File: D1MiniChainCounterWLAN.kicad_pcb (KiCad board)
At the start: 2 copper layers, 74.9 x 50.2 mm, 20 parts, among them J1 Power, J2 D24V10F5, J3 Chain Sens., J4 Chain Sw., K1 G5Q-1A, K2 G5Q-1A, Q1 BC337, Q2 BC337, Q3 BC337, Q4 BC337, U1 WeMos_D1_mini, U2 H11L1

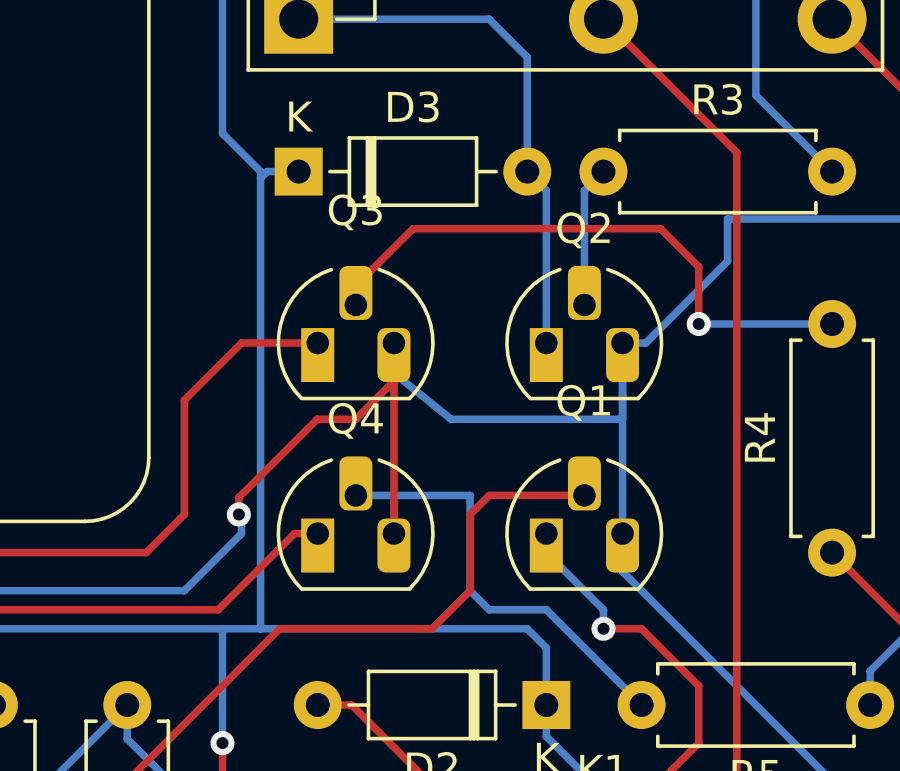
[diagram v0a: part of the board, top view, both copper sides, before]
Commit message: Version 1.1
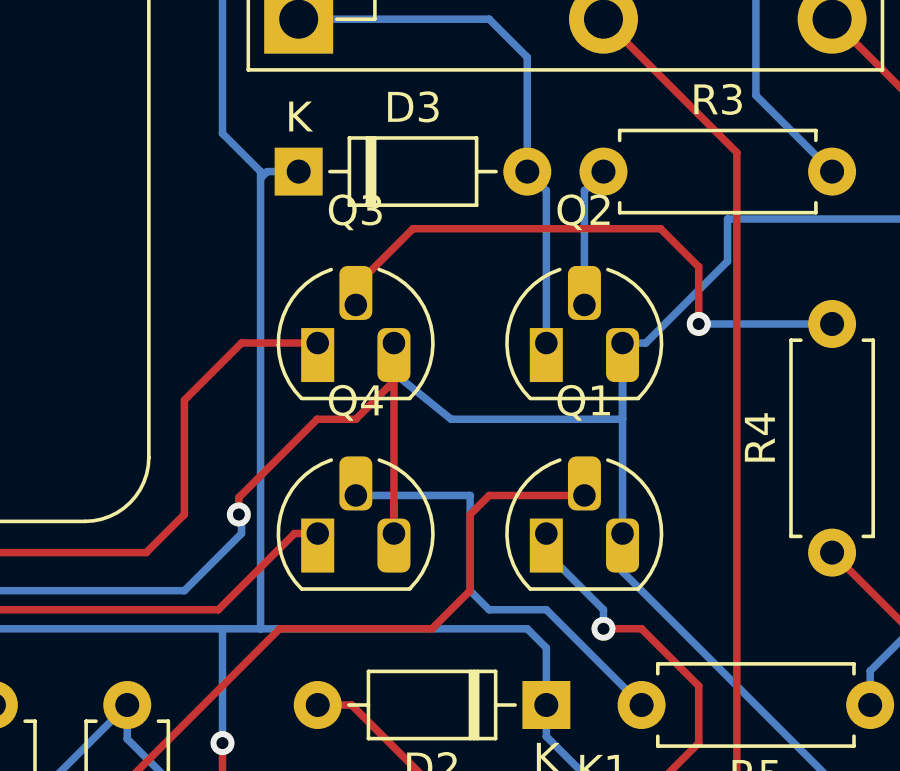
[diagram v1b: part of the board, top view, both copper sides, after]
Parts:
- Q2, Q4: footprint Package_TO_SOT_THT:TO-92L_HandSolder -> Package_TO_SOT_THT:TO-92_HandSolder
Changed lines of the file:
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@@
+  )
+  (module Package_TO_SOT_THT:TO-92_HandSolder (layer F.Cu)
+    (at 137.16 76.835)
+    (descr "TO-92 leads molded, narrow, drill 0.75mm, handsoldering variant with enlarged pads (see NXP sot054_po.pdf)")
+    (tags "to-92 sc-43 sc-43a sot54 PA33 transistor")
+    (fp_text reference Q4 (at 1.27 -4.4) (layer F.SilkS)
+      (effects (font (size 1 1) (thickness 0.15)))
+    )
+    (fp_text value BC337 (at 1.27 2.79) (layer F.Fab)
+      (effects (font (size 1 1) (thickness 0.15)))
+    )
+    (fp_arc (start 1.27 0) (end 2.05 -2.45) (angle 117.6433766) (layer F.SilkS) (width 0.12))
+    (fp_arc (start 1.27 0) (end 1.27 -2.48) (angle -135) (layer F.Fab) (width 0.1))
+    (fp_arc (start 1.27 0) (end 0.45 -2.45) (angle -116.9632683) (layer F.SilkS) (width 0.12))
+    (fp_arc (start 1.27 0) (end 1.27 -2.48) (angle 135) (layer F.Fab) (width 0.1))
+    (fp_line (start 4 2.01) (end -1.46 2.01) (layer F.CrtYd) (width 0.05))
+    (fp_line (start 4 2.01) (end 4 -3.05) (layer F.CrtYd) (width 0.05))
+    (fp_line (start -1.45 -3.05) (end -1.46 2.01) (layer F.CrtYd) (width 0.05))
+    (fp_line (start -1.46 -3.05) (end 4 -3.05) (layer F.CrtYd) (width 0.05))
+    (fp_line (start -0.5 1.75) (end 3 1.75) (layer F.Fab) (width 0.1))
+    (fp_line (start -0.53 1.85) (end 3.07 1.85) (layer F.SilkS) (width 0.12))
+    (fp_text user %R (at 1.27 -4.4) (layer F.Fab)
+      (effects (font (size 1 1) (thickness 0.15)))
+    )
+    (pad 1 thru_hole rect (at 0 0) (size 1.1 1.8) (drill 0.75 (offset 0 0.4)) (layers *.Cu *.Mask)
+      (net 11 "Net-(Q4-Pad1)"))
+    (pad 3 thru_hole roundrect (at 2.54 0) (size 1.1 1.8) (drill 0.75 (offset 0 0.4)) (layers *.Cu *.Mask) (roundrect_rratio 0.25)
+      (net 18 GND))
+    (pad 2 thru_hole roundrect (at 1.27 -1.27) (size 1.1 1.8) (drill 0.75 (offset 0 -0.4)) (layers *.Cu *.Mask) (roundrect_rratio 0.25)
+      (net 12 "Net-(Q4-Pad2)"))
+    (model ${KISYS3DMOD}/Package_TO_SOT_THT.3dshapes/TO-92.wrl
+      (at (xyz 0 0 0))
+      (scale (xyz 1 1 1))
+      (rotate (xyz 0 0 0))
+    )
+  )
+  (module Package_TO_SOT_THT:TO-92_HandSolder (layer F.Cu)
+    (at 144.78 70.485)
+    (descr "TO-92 leads molded, narrow, drill 0.75mm, handsoldering variant with enlarged pads (see NXP sot054_po.pdf)")
+    (tags "to-92 sc-43 sc-43a sot54 PA33 transistor")
+    (fp_text reference Q2 (at 1.27 -4.4) (layer F.SilkS)
+      (effects (font (size 1 1) (thickness 0.15)))
+    )
+    (fp_text value BC337 (at 1.27 2.79) (layer F.Fab)
+      (effects (font (size 1 1) (thickness 0.15)))
+    )
+    (fp_arc (start 1.27 0) (end 2.05 -2.45) (angle 117.6433766) (layer F.SilkS) (width 0.12))
+    (fp_arc (start 1.27 0) (end 1.27 -2.48) (angle -135) (layer F.Fab) (width 0.1))
+    (fp_arc (start 1.27 0) (end 0.45 -2.45) (angle -116.9632683) (layer F.SilkS) (width 0.12))
+    (fp_arc (start 1.27 0) (end 1.27 -2.48) (angle 135) (layer F.Fab) (width 0.1))
+    (fp_line (start 4 2.01) (end -1.46 2.01) (layer F.CrtYd) (width 0.05))
+    (fp_line (start 4 2.01) (end 4 -3.05) (layer F.CrtYd) (width 0.05))
+    (fp_line (start -1.45 -3.05) (end -1.46 2.01) (layer F.CrtYd) (width 0.05))
+    (fp_line (start -1.46 -3.05) (end 4 -3.05) (layer F.CrtYd) (width 0.05))
+    (fp_line (start -0.5 1.75) (end 3 1.75) (layer F.Fab) (width 0.1))
+    (fp_line (start -0.53 1.85) (end 3.07 1.85) (layer F.SilkS) (width 0.12))
+    (fp_text user %R (at 1.27 -4.4) (layer F.Fab)
+      (effects (font (size 1 1) (thickness 0.15)))
+    )
+    (pad 1 thru_hole rect (at 0 0) (size 1.1 1.8) (drill 0.75 (offset 0 0.4)) (layers *.Cu *.Mask)
+      (net 3 "Net-(D3-Pad2)"))
+    (pad 3 thru_hole roundrect (at 2.54 0) (size 1.1 1.8) (drill 0.75 (offset 0 0.4)) (layers *.Cu *.Mask) (roundrect_rratio 0.25)
+      (net 18 GND))
+    (pad 2 thru_hole roundrect (at 1.27 -1.27) (size 1.1 1.8) (drill 0.75 (offset 0 -0.4)) (layers *.Cu *.Mask) (roundrect_rratio 0.25)
+      (net 8 "Net-(Q2-Pad2)"))
+    (model ${KISYS3DMOD}/Package_TO_SOT_THT.3dshapes/TO-92.wrl
+      (at (xyz 0 0 0))
+      (scale (xyz 1 1 1))
+      (rotate (xyz 0 0 0))
+    )
   )
   (module Package_TO_SOT_THT:TO-92_HandSolder (layer F.Cu)
@@
       (at (xyz 0 0 0))
       (scale (xyz 1 1 1))
-      (rotate (xyz 0 0 0))
-    )
-  )
-  (module Package_TO_SOT_THT:TO-92L_HandSolder (layer F.Cu)
-    (at 137.16 76.835)
-    (descr "TO-92L leads in-line (large body variant of TO-92), also known as TO-226, wide, drill 0.75mm, hand-soldering variant with enlarged pads (see https://www.diodes.com/assets/Package-Files/TO92L.pdf and http://www.ti.com/lit/an/snoa059/snoa059.pdf)")
-    (tags "to-92 sc-43 sc-43a sot54 PA33 transistor")
-    (fp_text reference Q4 (at 1.27 -3.8) (layer F.SilkS)
-      (effects (font (size 1 1) (thickness 0.15)))
-    )
-    (fp_text value BC337 (at 1.27 2.79) (layer F.Fab)
-      (effects (font (size 1 1) (thickness 0.15)))
-    )
-    (fp_arc (start 1.27 0) (end 2.05 -2.45) (angle 117.6433766) (layer F.SilkS) (width 0.12))
-    (fp_arc (start 1.27 0) (end 1.27 -2.48) (angle -135) (layer F.Fab) (width 0.1))
-    (fp_arc (start 1.27 0) (end 0.45 -2.45) (angle -116.9763941) (layer F.SilkS) (width 0.12))
-    (fp_arc (start 1.27 0) (end 1.27 -2.48) (angle 135) (layer F.Fab) (width 0.1))
-    (fp_line (start 4 2.01) (end -1.46 2.01) (layer F.CrtYd) (width 0.05))
-    (fp_line (start 4 2.01) (end 4 -3.05) (layer F.CrtYd) (width 0.05))
-    (fp_line (start -1.45 -3.05) (end -1.46 2.01) (layer F.CrtYd) (width 0.05))
-    (fp_line (start -1.46 -3.05) (end 4 -3.05) (layer F.CrtYd) (width 0.05))
-    (fp_line (start -0.5 1.75) (end 3 1.75) (layer F.Fab) (width 0.1))
-    (fp_line (start -0.53 1.85) (end 3.07 1.85) (layer F.SilkS) (width 0.12))
-    (fp_text user %R (at 1.27 0) (layer F.Fab)
-      (effects (font (size 1 1) (thickness 0.15)))
-    )
-    (pad 1 thru_hole rect (at 0 0) (size 1.1 1.8) (drill 0.75 (offset 0 0.4)) (layers *.Cu *.Mask)
-      (net 11 "Net-(Q4-Pad1)"))
-    (pad 3 thru_hole roundrect (at 2.54 0) (size 1.1 1.8) (drill 0.75 (offset 0 0.4)) (layers *.Cu *.Mask) (roundrect_rratio 0.25)
-      (net 18 GND))
-    (pad 2 thru_hole roundrect (at 1.27 -1.27) (size 1.1 1.8) (drill 0.75 (offset 0 -0.4)) (layers *.Cu *.Mask) (roundrect_rratio 0.25)
-      (net 12 "Net-(Q4-Pad2)"))
-    (model ${KISYS3DMOD}/Package_TO_SOT_THT.3dshapes/TO-92L.wrl
-      (at (xyz 0 0 0))
-      (scale (xyz 1 1 1))
-      (rotate (xyz 0 0 0))
-    )
-  )
-  (module Package_TO_SOT_THT:TO-92L_HandSolder (layer F.Cu)
-    (at 144.78 70.485)
-    (descr "TO-92L leads in-line (large body variant of TO-92), also known as TO-226, wide, drill 0.75mm, hand-soldering variant with enlarged pads (see https://www.diodes.com/assets/Package-Files/TO92L.pdf and http://www.ti.com/lit/an/snoa059/snoa059.pdf)")
-    (tags "to-92 sc-43 sc-43a sot54 PA33 transistor")
-    (fp_text reference Q2 (at 1.27 -3.8) (layer F.SilkS)
-      (effects (font (size 1 1) (thickness 0.15)))
-    )
-    (fp_text value BC337 (at 1.27 2.79) (layer F.Fab)
-      (effects (font (size 1 1) (thickness 0.15)))
-    )
-    (fp_arc (start 1.27 0) (end 2.05 -2.45) (angle 117.6433766) (layer F.SilkS) (width 0.12))
-    (fp_arc (start 1.27 0) (end 1.27 -2.48) (angle -135) (layer F.Fab) (width 0.1))
-    (fp_arc (start 1.27 0) (end 0.45 -2.45) (angle -116.9763941) (layer F.SilkS) (width 0.12))
-    (fp_arc (start 1.27 0) (end 1.27 -2.48) (angle 135) (layer F.Fab) (width 0.1))
-    (fp_line (start 4 2.01) (end -1.46 2.01) (layer F.CrtYd) (width 0.05))
-    (fp_line (start 4 2.01) (end 4 -3.05) (layer F.CrtYd) (width 0.05))
-    (fp_line (start -1.45 -3.05) (end -1.46 2.01) (layer F.CrtYd) (width 0.05))
-    (fp_line (start -1.46 -3.05) (end 4 -3.05) (layer F.CrtYd) (width 0.05))
-    (fp_line (start -0.5 1.75) (end 3 1.75) (layer F.Fab) (width 0.1))
-    (fp_line (start -0.53 1.85) (end 3.07 1.85) (layer F.SilkS) (width 0.12))
-    (fp_text user %R (at 1.27 0) (layer F.Fab)
-      (effects (font (size 1 1) (thickness 0.15)))
-    )
-    (pad 1 thru_hole rect (at 0 0) (size 1.1 1.8) (drill 0.75 (offset 0 0.4)) (layers *.Cu *.Mask)
-      (net 3 "Net-(D3-Pad2)"))
-    (pad 3 thru_hole roundrect (at 2.54 0) (size 1.1 1.8) (drill 0.75 (offset 0 0.4)) (layers *.Cu *.Mask) (roundrect_rratio 0.25)
-      (net 18 GND))
-    (pad 2 thru_hole roundrect (at 1.27 -1.27) (size 1.1 1.8) (drill 0.75 (offset 0 -0.4)) (layers *.Cu *.Mask) (roundrect_rratio 0.25)
-      (net 8 "Net-(Q2-Pad2)"))
-    (model ${KISYS3DMOD}/Package_TO_SOT_THT.3dshapes/TO-92L.wrl
-      (at (xyz 0 0 0))
-      (scale (xyz 1 1 1))
